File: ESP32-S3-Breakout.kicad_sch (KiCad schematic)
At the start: 34 parts, among them J1 USB_C_Receptacle_USB2.0, J2 USB_C_Receptacle_USB2.0, J3 Conn_01x21, J4 Conn_01x21, Q1 Q_NPN_BCE, Q2 Q_NPN_BCE, SW1 SW_Push, SW2 SW_Push, U1 USBLC6-2SC6, U2 USBLC6-2SC6, U3 ESP32-S3-WROOM, U4 CH340C, U5 XC6210B332MR, Y1 32.768kHz

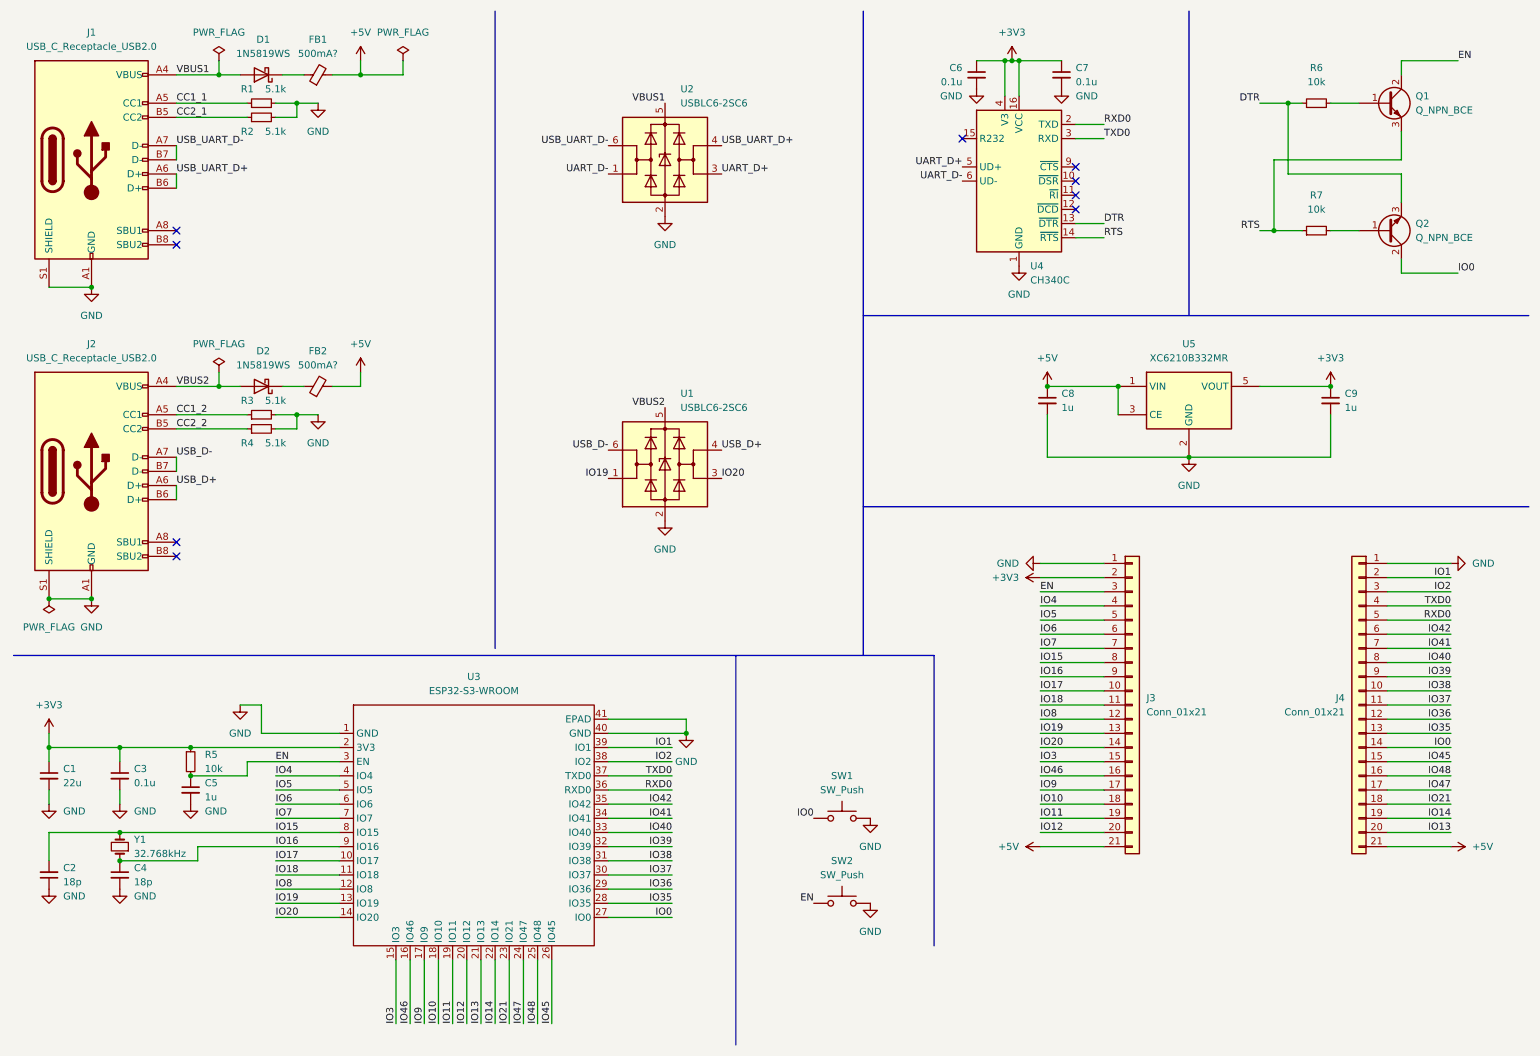
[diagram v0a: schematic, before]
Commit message: initial group of modifications.
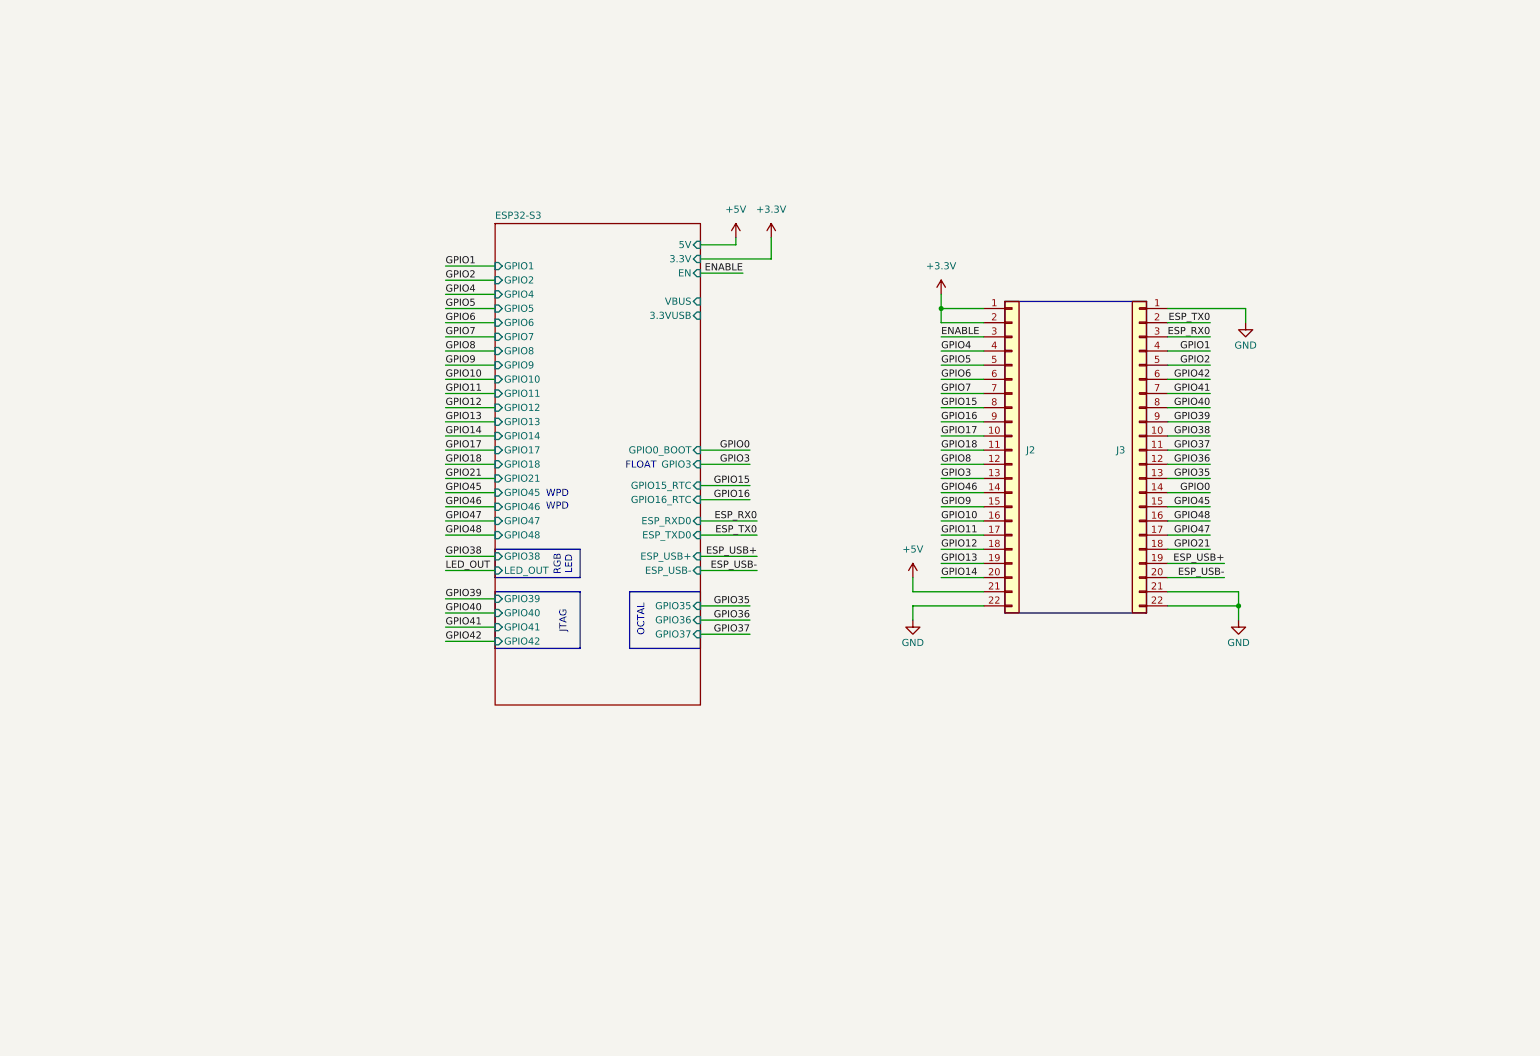
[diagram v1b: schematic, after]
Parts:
- removed C1: 22u, Capacitor_SMD:C_0805_2012Metric, symbol Device:C_Small
- removed C2, C4: 18p, Capacitor_SMD:C_0603_1608Metric, symbol Device:C_Small
- removed C3, C6, C7: 0.1u, Capacitor_SMD:C_0603_1608Metric, symbol Device:C_Small
- removed C5: 1u, Capacitor_SMD:C_0603_1608Metric, symbol Device:C_Small
- removed C8, C9: 1u, Capacitor_SMD:C_0805_2012Metric, symbol Device:C_Small
- removed D1, D2: 1N5819WS, Diode_SMD:D_SOD-323, symbol Diode:1N5819WS
- removed FB1, FB2: 500mA?, Inductor_SMD:L_0603_1608Metric, symbol Device:FerriteBead_Small
- removed J1, J2: USB_C_Receptacle_USB2.0, Connector_USB:USB_C_Receptacle_HRO_TYPE-C-31-M-12, symbol Connector:USB_C_Receptacle_USB2.0
- removed J3, J4: Conn_01x21, Connector_PinHeader_2.54mm:PinHeader_1x21_P2.54mm_Vertical, symbol Connector_Generic:Conn_01x21
- removed Q1, Q2: Q_NPN_BCE, Package_TO_SOT_SMD:SOT-23, symbol Device:Q_NPN_BCE
- removed R1, R2, R3, R4: 5.1k, Resistor_SMD:R_0603_1608Metric, symbol Device:R_Small
- removed R5, R6, R7: 10k, Resistor_SMD:R_0603_1608Metric, symbol Device:R_Small
- removed SW1, SW2: SW_Push, Button_Switch_SMD:SW_SPST_B3U-1000P, symbol Switch:SW_Push
- removed U1, U2: USBLC6-2SC6, Package_TO_SOT_SMD:SOT-23-6, symbol Power_Protection:USBLC6-2SC6
- removed U3: ESP32-S3-WROOM, RF_Module:ESP32-S3-WROOM-1, symbol ESP32-S3-Breakout:ESP32-S3-WROOM
- removed U4: CH340C, Package_SO:SOIC-16_3.9x9.9mm_P1.27mm, symbol Interface_USB:CH340C
- removed U5: XC6210B332MR, Package_TO_SOT_SMD:SOT-23-5, symbol Regulator_Linear:XC6210B332MR
- removed Y1: 32.768kHz, Crystal:Crystal_SMD_3215-2Pin_3.2x1.5mm, symbol Device:Crystal_Small
- added J2, J3: Conn_01x22, Connector_PinHeader_2.54mm:PinHeader_1x22_P2.54mm_Vertical, symbol Connector_Generic:Conn_01x22
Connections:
- net +5V: now also J2.21 (Pin_21)
- net GND: now also J2.22 (Pin_22), J3.1 (Pin_1), J3.21 (Pin_21), J3.22 (Pin_22)
- new net +3.3V: J2.1 (Pin_1), J2.2 (Pin_2)
- new net ENABLE: J2.3 (Pin_3)
- new net ESP_RX0: J3.3 (Pin_3)
- new net ESP_TX0: J3.2 (Pin_2)
- new net ESP_USB+: J3.19 (Pin_19)
- new net ESP_USB-: J3.20 (Pin_20)
- new net GPIO0: J3.14 (Pin_14)
- new net GPIO1: J3.4 (Pin_4)
- new net GPIO10: J2.16 (Pin_16)
- new net GPIO11: J2.17 (Pin_17)
- new net GPIO12: J2.18 (Pin_18)
- new net GPIO13: J2.19 (Pin_19)
- new net GPIO14: J2.20 (Pin_20)
- new net GPIO15: J2.8 (Pin_8)
- new net GPIO16: J2.9 (Pin_9)
- new net GPIO17: J2.10 (Pin_10)
- new net GPIO18: J2.11 (Pin_11)
- new net GPIO2: J3.5 (Pin_5)
- new net GPIO21: J3.18 (Pin_18)
- new net GPIO3: J2.13 (Pin_13)
- new net GPIO35: J3.13 (Pin_13)
- new net GPIO36: J3.12 (Pin_12)
- new net GPIO37: J3.11 (Pin_11)
- new net GPIO38: J3.10 (Pin_10)
- new net GPIO39: J3.9 (Pin_9)
- new net GPIO4: J2.4 (Pin_4)
- new net GPIO40: J3.8 (Pin_8)
- new net GPIO41: J3.7 (Pin_7)
- new net GPIO42: J3.6 (Pin_6)
- new net GPIO45: J3.15 (Pin_15)
- new net GPIO46: J2.14 (Pin_14)
- new net GPIO47: J3.17 (Pin_17)
- new net GPIO48: J3.16 (Pin_16)
- new net GPIO5: J2.5 (Pin_5)
- new net GPIO6: J2.6 (Pin_6)
- new net GPIO7: J2.7 (Pin_7)
- new net GPIO8: J2.12 (Pin_12)
- new net GPIO9: J2.15 (Pin_15)
- no-connect marks 9 -> 0
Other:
- added sheet ESP32-S3 (esp32-s3.kicad_sch)
- note added: "FLOAT"
- note added: "JTAG"
- note added: "OCTAL"
- note added: "RGB LED"
- note added: "WPD"
